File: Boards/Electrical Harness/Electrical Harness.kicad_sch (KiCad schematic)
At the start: 4 parts, among them J1 10-18-1041, J2 39-28-8080, J3 39-28-8080, J4 10-18-1041

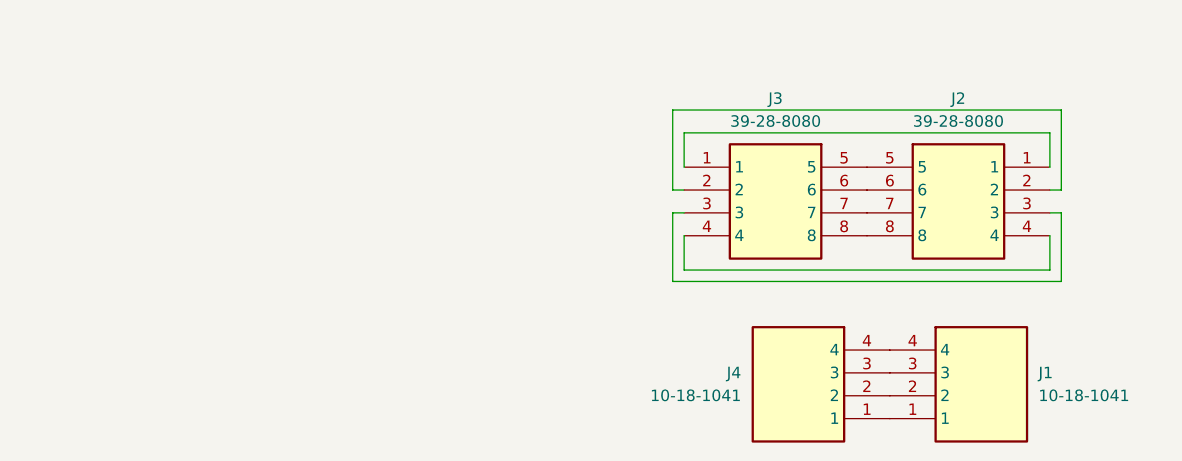
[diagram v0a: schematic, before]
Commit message: PCB CALHA
PCB CALHA
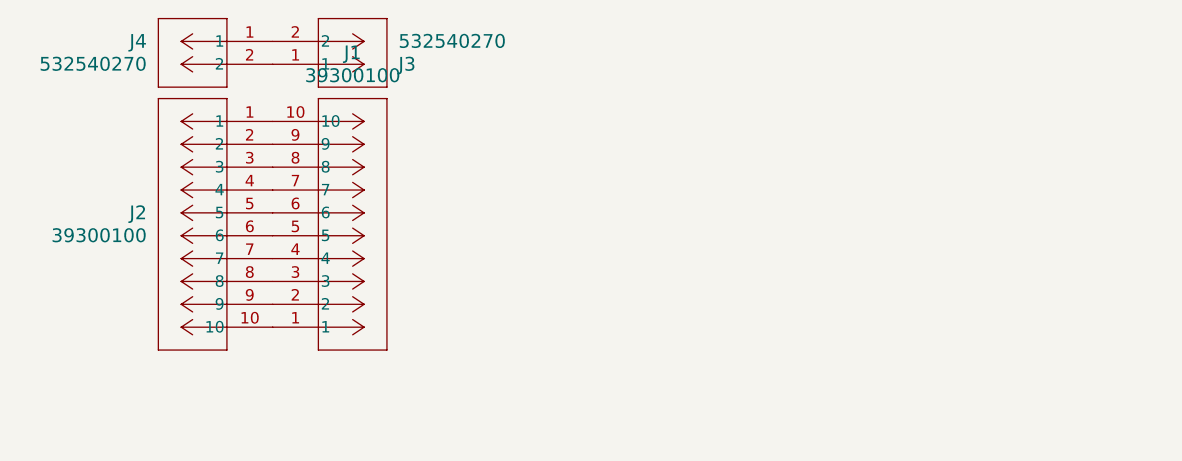
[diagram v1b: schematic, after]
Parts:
- removed J1, J4: 10-18-1041, 10181041, symbol 10-18-1041:10-18-1041
- removed J2, J3: 39-28-8080, 39-28-8080, symbol 39-28-8080:39-28-8080
- added J1, J2: 39300100, CONN_5569-10A_MOL, symbol 2025-09-29_18-23-06:39300100
- added J3, J4: 532540270, CONN02_532540270_MOL, symbol 2025-09-29_18-42-02:532540270
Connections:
- new net: J1.1, J2.10
- new net: J1.10, J2.1
- new net: J1.2, J2.9
- new net: J1.3, J2.8
- new net: J1.4, J2.7
- new net: J1.5, J2.6
- new net: J1.6, J2.5
- new net: J1.7, J2.4
- new net: J1.8, J2.3
- new net: J1.9, J2.2
- new net: J3.1, J4.2
- new net: J3.2, J4.1
